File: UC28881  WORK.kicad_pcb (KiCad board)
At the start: 2 copper layers, 102 x 50 mm, 22 parts, among them J1 Screw_Terminal_01x02, J2 Screw_Terminal_01x02, U1 UCC28881

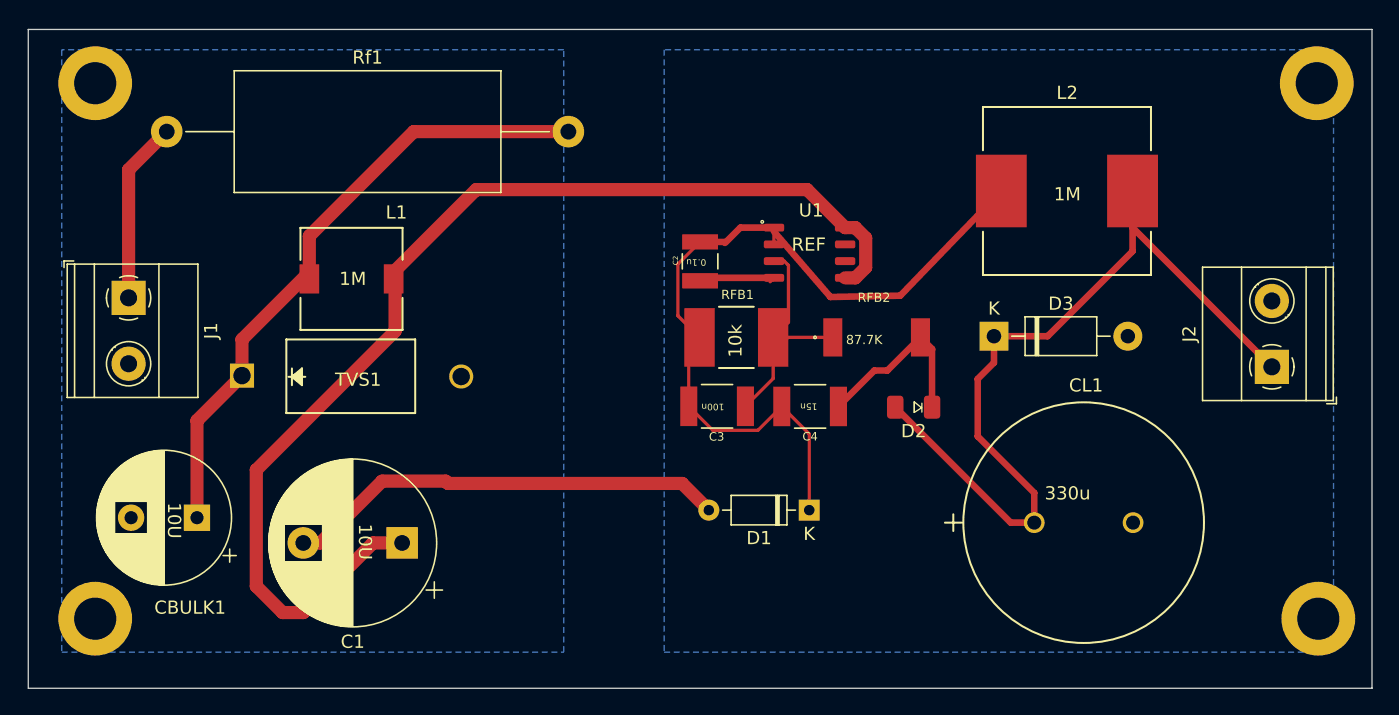
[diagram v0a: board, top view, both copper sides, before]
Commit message: Updated PCB
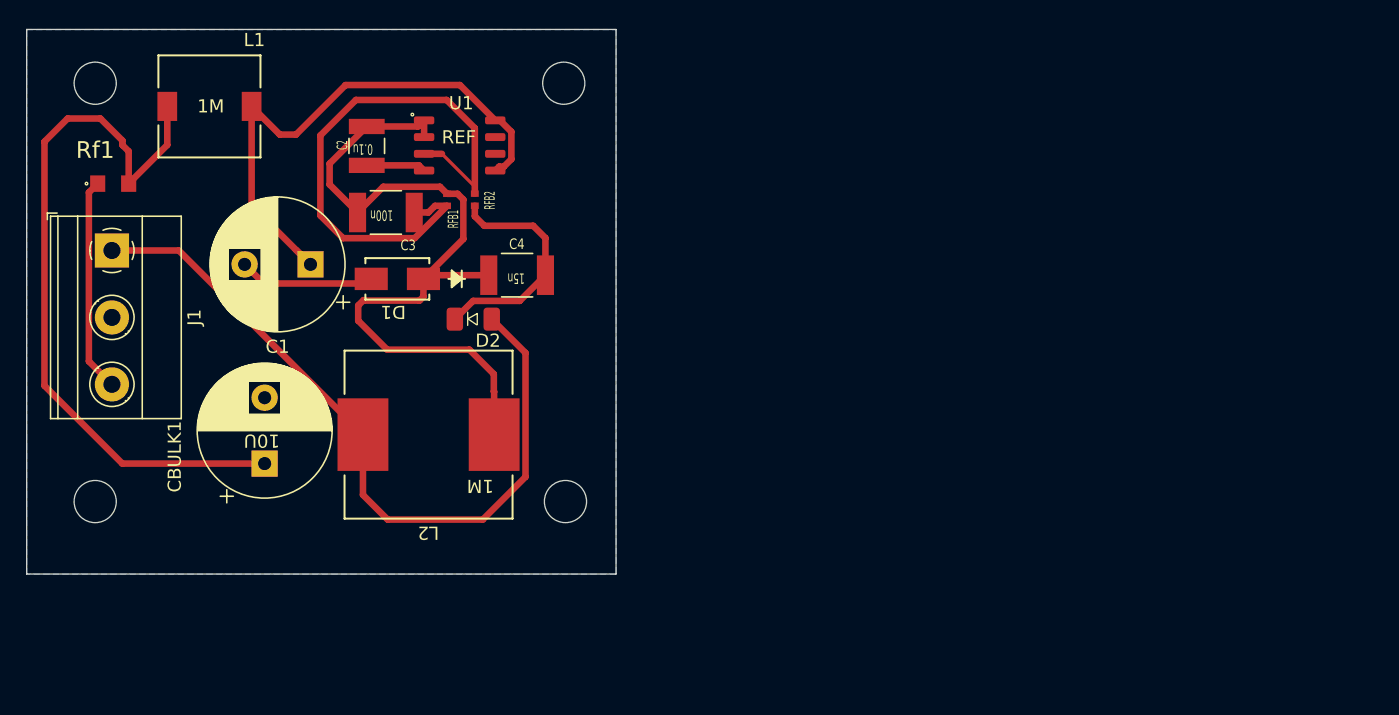
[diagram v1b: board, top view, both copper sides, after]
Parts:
- removed CL1: 330u, CL1:CAP_UAQ_18X20_NCH
- removed D3: 1N5819, Diode_THT:D_DO-41_SOD81_P10.16mm_Horizontal
- removed J2: Screw_Terminal_01x02, TerminalBlock_Phoenix:TerminalBlock_Phoenix_MKDS-1,5-2_1x02_P5.00mm_Horizontal
- removed REF** (x4): MountingHole_3.2mm_M3_DIN965_Pad, MountingHole:MountingHole_3.2mm_M3_DIN965_Pad
- removed TVS1: D_Zener, TVS1:1.5KESeries_LTF
- added H1: MountingHole, MountingHole:MountingHole_3.2mm_M3_DIN965, F.Cu at (76.2, 69.8)
- added H2: MountingHole, MountingHole:MountingHole_3.2mm_M3_DIN965, F.Cu at (111.9, 69.8)
- added H3: MountingHole, MountingHole:MountingHole_3.2mm_M3_DIN965, F.Cu at (111.8, 38.1)
- added H4: MountingHole, MountingHole:MountingHole_3.2mm_M3_DIN965, F.Cu at (76.2, 38.1)
- C1: footprint Capacitor_THT:CP_Radial_D12.5mm_P7.50mm -> Capacitor_THT:CP_Radial_D10.0mm_P5.00mm
- D1: footprint Diode_THT:D_DO-35_SOD27_P7.62mm_Horizontal -> D1:SMA_STM-M
- D2: value SS1P3L -> M7; footprint Diode_SMD:D_1206_3216Metric -> D2:D2
- J1: value Screw_Terminal_01x02 -> Screw_Terminal_01x03; footprint TerminalBlock_Phoenix:TerminalBlock_Phoenix_MKDS-1,5-2_1x02_P5.00mm_Horizontal -> TerminalBlock_Phoenix:TerminalBlock_Phoenix_MKDS-1,5-3-5.08_1x03_P5.08mm_Horizontal
- RFB1: footprint 10k resistor:10k RES_3540_TEC-M -> 10k resistor:10k RESC1005X35N
- RFB2: value 87.7K -> 110k; footprint 88.7k resistor:ERJS1T_U1T__2512_ -> 110k resistor:110k RESC1005X35N
- Rf1: footprint Resistor_THT:R_Axial_DIN0922_L20.0mm_D9.0mm_P30.48mm_Horizontal -> RF:ERJUP6
- moved L2 51.9 mm to (101.5, 64.8), turned to 180 degrees
- moved D1 35.8 mm to (99.1, 53.0)
- moved D2 34.2 mm to (104.8, 55.9), turned to 0 degrees
- moved RFB2 32.2 mm to (105.0, 46.9), turned to -90 degrees
- moved C3 29.1 mm to (98.3, 47.9)
- moved U1 27.8 mm to (103.8, 42.8)
- moved C2 26.8 mm to (96.8, 42.9)
- moved C4 24.4 mm to (108.2, 52.7)
- moved RFB1 24.3 mm to (102.9, 47.0), turned to -90 degrees
- moved C1 22.3 mm to (92.5, 51.9)
- moved L1 17.0 mm to (84.9, 39.9)
- moved CBULK1 6.58 mm to (89.1, 67.0), turned to 90 degrees
- moved Rf1 5.66 mm to (77.6, 45.7)
- moved J1 3.81 mm to (77.5, 50.8)
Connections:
- J1 pad 1: /HV_IN_P -> /10V_OUT_P
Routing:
- net Net-(U1-DRAIN): track 86.3 -> 43.5 mm
- net /Feedback pin: track 17.8 -> 44.2 mm
- net /GND: track 33.6 -> 10.4 mm
- net /10V_OUT_P: track 66.1 -> 56.9 mm
- net Net-(CBULK1-Pad1): track 48.5 -> 55.6 mm
- net Net-(D2-K): track 14.6 -> 17.9 mm
- net /HV_IN_P: track 13.8 -> 16.2 mm
- net Net-(D1-K): track 62.1 -> 60.3 mm
- net Net-(U1-VDD): track 6.12 -> 4.51 mm
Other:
- board size 102 x 50 mm -> 44.7 x 41.3 mm
